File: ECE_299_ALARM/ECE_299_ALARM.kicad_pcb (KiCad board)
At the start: 2 copper layers, 60 x 50 mm, 16 parts, among them SW1 SW_Push_Dual, SW2 SW_Push_Dual, SW3 SW_Push_Dual, SW4 SW_Push_Dual, U1 RDA5807M_Module, U2 RPi_Pico_TH, U3 LM386

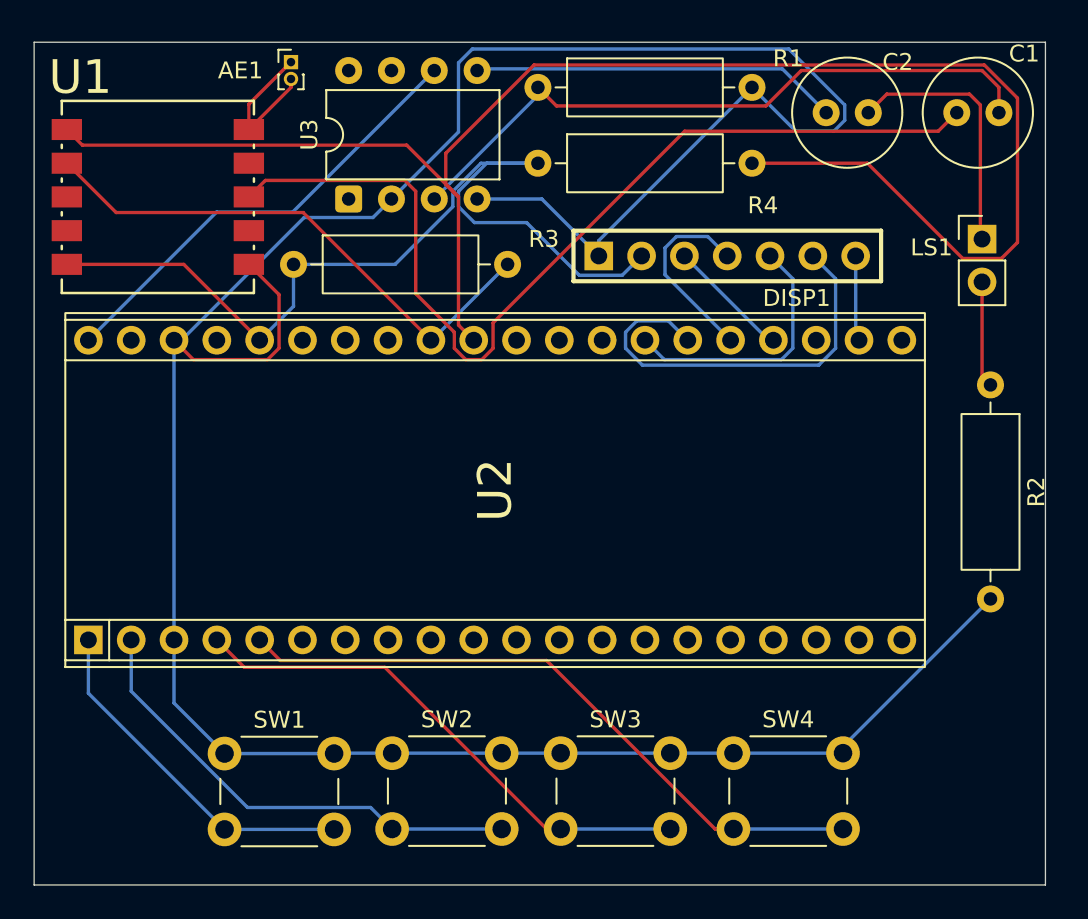
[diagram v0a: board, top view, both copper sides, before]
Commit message: added pcb files
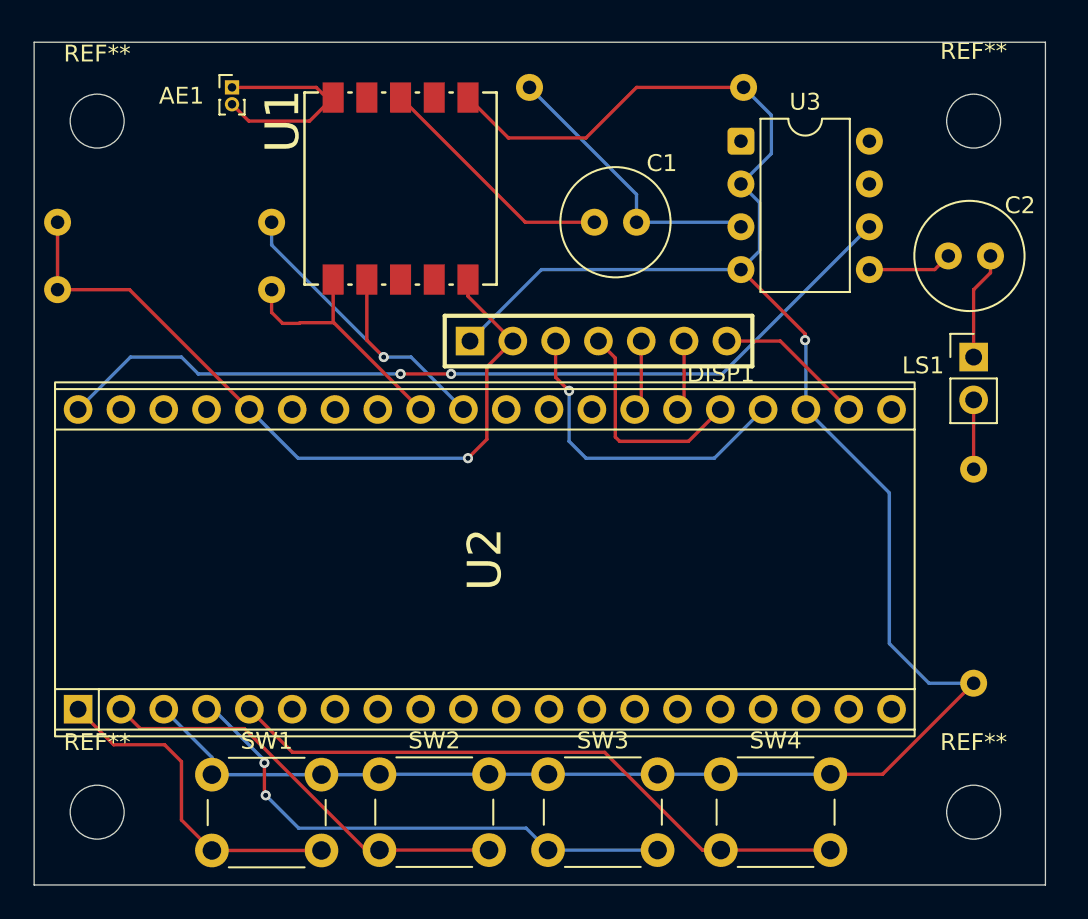
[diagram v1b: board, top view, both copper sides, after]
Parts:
- added REF**: MountingHole_3.2mm_M3, MountingHole:MountingHole_3.2mm_M3, F.Cu at (90.0, 115.0)
- added REF**: MountingHole_3.2mm_M3, MountingHole:MountingHole_3.2mm_M3, F.Cu at (142.0, 115.0)
- added REF**: MountingHole_3.2mm_M3, MountingHole:MountingHole_3.2mm_M3, F.Cu at (142.0, 74.0)
- added REF**: MountingHole_3.2mm_M3, MountingHole:MountingHole_3.2mm_M3, F.Cu at (90.0, 74.0)
- R1, R2, R3, R4: moved to B.Cu
- moved R4 28.7 mm to (87.7, 80.0)
- moved U3 23.5 mm to (128.2, 75.2), turned to 0 degrees
- moved C1 22.5 mm to (119.5, 80.0)
- moved U1 14.4 mm to (108.0, 78.0), turned to 90 degrees
- moved R3 14.1 mm to (87.7, 84.0)
- moved C2 11.2 mm to (140.5, 82.0)
- moved DISP1 9.16 mm to (102.0, 119.0)
- moved LS1 7.02 mm to (142.0, 88.0)
- moved R2 5.10 mm to (142.0, 94.7)
- moved U2 4.16 mm to (113.0, 100.0)
- moved AE1 3.81 mm to (98.0, 72.0)
- moved SW1 1.46 mm to (96.8, 112.8)
- moved SW2 1.46 mm to (106.8, 112.8)
- moved SW3 1.46 mm to (116.8, 112.8)
- moved SW4 1.46 mm to (127.0, 112.8)
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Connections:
- R3 pad 2: Net-(U1-SCLK) -> Net-(U1-SDIO)
- R4 pad 2: Net-(U1-SDIO) -> Net-(U1-SCLK)
- U2 pad 23: unconnected-(U2-GND-Pad23) -> GND
- U2 pad 31: Net-(U1-SDIO) -> Net-(U1-SCLK)
- U2 pad 32: Net-(U1-SCLK) -> Net-(U1-SDIO)
- U2 pad 38: GND -> unconnected-(U2-GND-Pad38)
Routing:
- net Net-(U1-SDIO): track 100.6 -> 15.2 mm
- net Net-(U1-LOUT): track 57.9 -> 14.6 mm
- net GND: track 168.8 -> 133.9 mm, vias 0 -> 1
- net +5V: track 27.1 -> 52.3 mm, vias 0 -> 2
- net Net-(U3-+): track 40.8 -> 16.9 mm
- net Net-(DISP1-DC): track 24.7 -> 4.22 mm
- net Net-(C2-Pad1): track 21.8 -> 5.02 mm
- net Net-(DISP1-SCLK): track 7.35 -> 19.4 mm, vias 0 -> 1
- net Net-(DISP1-RES): track 15.6 -> 4.22 mm
- net Net-(U1-SCLK): track 32.4 -> 21.8 mm, vias 0 -> 1
- net +3.3V: track 55.5 -> 45.3 mm, vias 0 -> 1
- net Net-(C2-Pad2): track 15.4 -> 6.41 mm
- net Net-(U1-FMIN): track 9.07 -> 13.2 mm
- net Net-(DISP1-CS): track 5.08 -> 8.91 mm
- net SW2: track 28.4 -> 25.3 mm
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
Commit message: Revert "Web app"
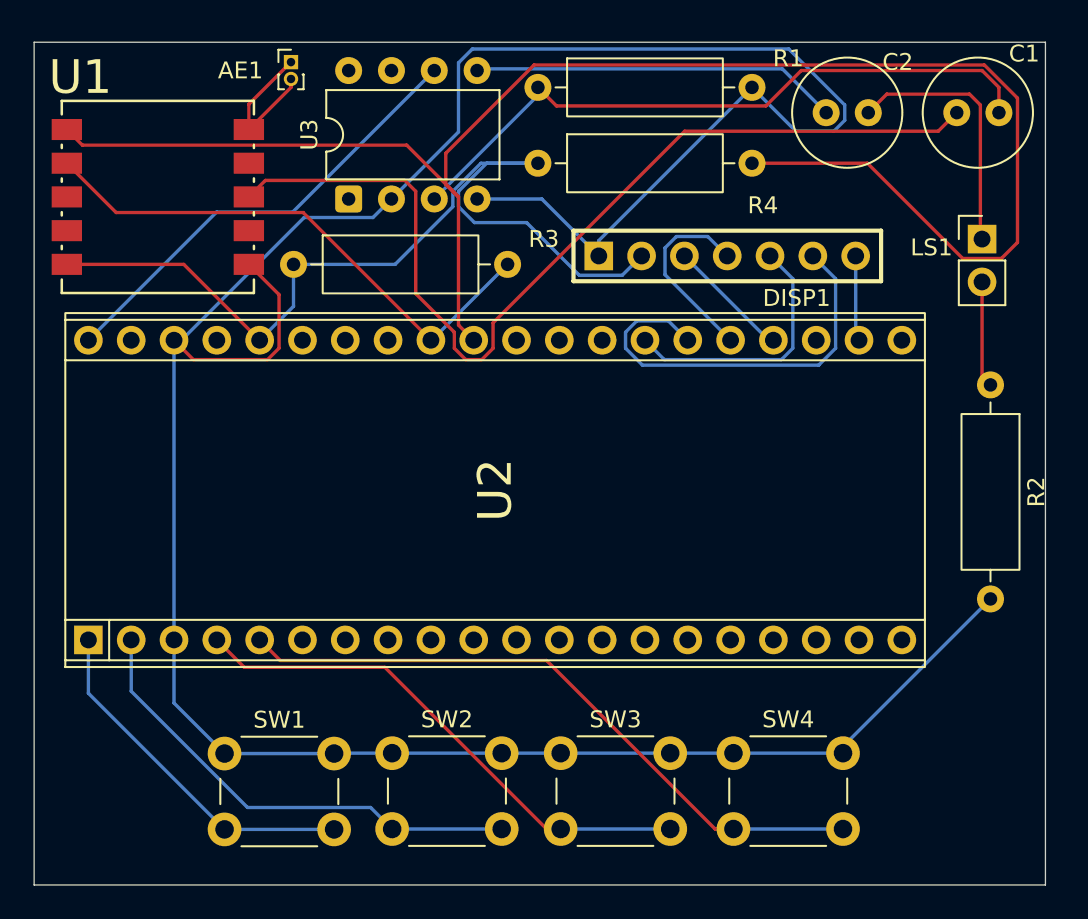
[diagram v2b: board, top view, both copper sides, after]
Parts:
- removed REF** (x4): MountingHole_3.2mm_M3, MountingHole:MountingHole_3.2mm_M3
- R1, R2, R3, R4: moved to F.Cu
- moved R4 28.7 mm to (116.2, 76.5)
- moved U3 23.5 mm to (104.9, 78.6), turned to 90 degrees
- moved C1 22.5 mm to (141.0, 73.5)
- moved U1 14.4 mm to (93.6, 78.5), turned to 0 degrees
- moved R3 14.1 mm to (101.7, 82.5)
- moved C2 11.2 mm to (133.2, 73.5)
- moved DISP1 9.16 mm to (109.6, 114.0)
- moved LS1 7.02 mm to (142.5, 81.0)
- moved R2 5.10 mm to (143.0, 89.7)
- moved U2 4.16 mm to (113.6, 95.9)
- moved AE1 3.81 mm to (101.5, 70.5)
- moved SW1 1.46 mm to (97.6, 111.5)
- moved SW2 1.46 mm to (107.5, 111.5)
- moved SW3 1.46 mm to (117.5, 111.5)
- moved SW4 1.46 mm to (127.8, 111.5)
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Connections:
- R3 pad 2: Net-(U1-SDIO) -> Net-(U1-SCLK)
- R4 pad 2: Net-(U1-SCLK) -> Net-(U1-SDIO)
- U2 pad 23: GND -> unconnected-(U2-GND-Pad23)
- U2 pad 31: Net-(U1-SCLK) -> Net-(U1-SDIO)
- U2 pad 32: Net-(U1-SDIO) -> Net-(U1-SCLK)
- U2 pad 38: unconnected-(U2-GND-Pad38) -> GND
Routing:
- net Net-(U1-SDIO): track 15.2 -> 100.6 mm
- net Net-(U1-LOUT): track 14.6 -> 57.9 mm
- net GND: track 133.9 -> 168.8 mm, vias 1 -> 0
- net +5V: track 52.3 -> 27.1 mm, vias 2 -> 0
- net Net-(U3-+): track 16.9 -> 40.8 mm
- net Net-(DISP1-DC): track 4.22 -> 24.7 mm
- net Net-(C2-Pad1): track 5.02 -> 21.8 mm
- net Net-(DISP1-SCLK): track 19.4 -> 7.35 mm, vias 1 -> 0
- net Net-(DISP1-RES): track 4.22 -> 15.6 mm
- net Net-(U1-SCLK): track 21.8 -> 32.4 mm, vias 1 -> 0
- net +3.3V: track 45.3 -> 55.5 mm, vias 1 -> 0
- net Net-(C2-Pad2): track 6.41 -> 15.4 mm
- net Net-(U1-FMIN): track 13.2 -> 9.07 mm
- net Net-(DISP1-CS): track 8.91 -> 5.08 mm
- net SW2: track 25.3 -> 28.4 mm
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
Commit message: Add files via upload
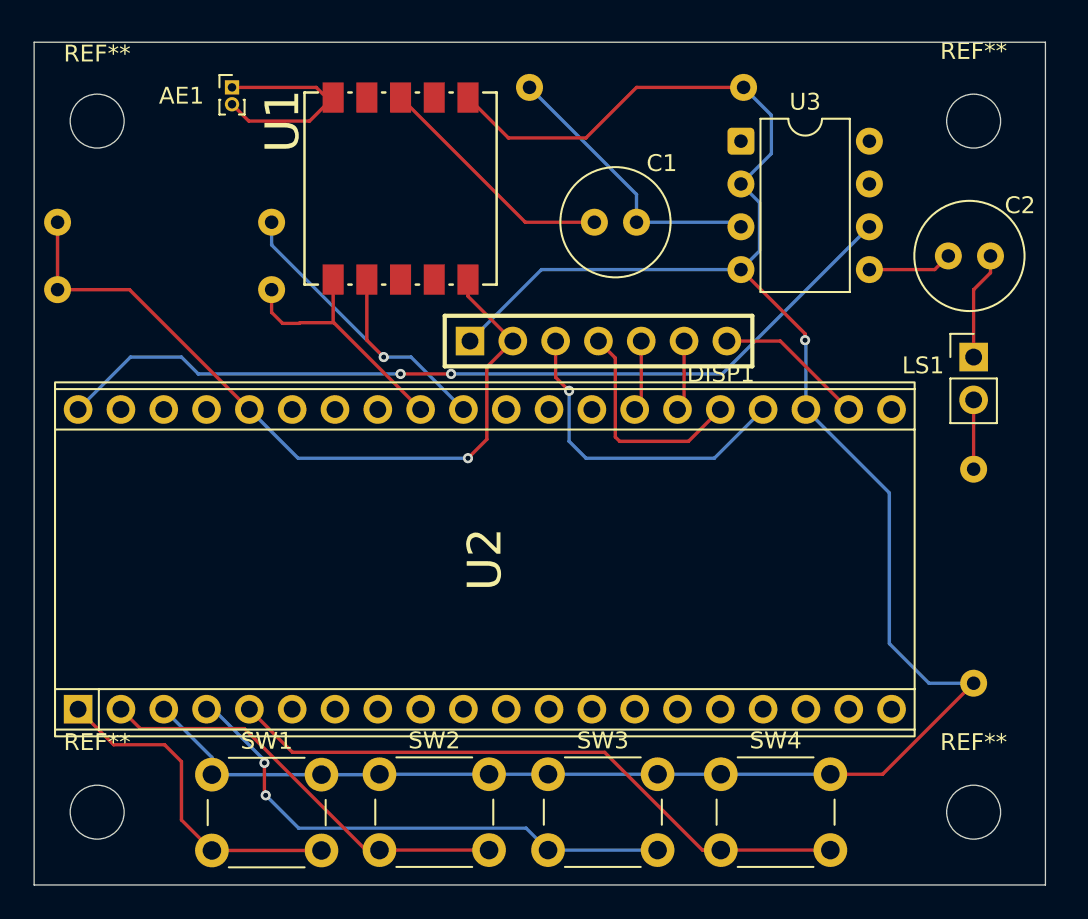
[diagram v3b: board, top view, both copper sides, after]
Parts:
- added REF**: MountingHole_3.2mm_M3, MountingHole:MountingHole_3.2mm_M3, F.Cu at (90.0, 115.0)
- added REF**: MountingHole_3.2mm_M3, MountingHole:MountingHole_3.2mm_M3, F.Cu at (142.0, 115.0)
- added REF**: MountingHole_3.2mm_M3, MountingHole:MountingHole_3.2mm_M3, F.Cu at (142.0, 74.0)
- added REF**: MountingHole_3.2mm_M3, MountingHole:MountingHole_3.2mm_M3, F.Cu at (90.0, 74.0)
- R1, R2, R3, R4: moved to B.Cu
- moved R4 28.7 mm to (87.7, 80.0)
- moved U3 23.5 mm to (128.2, 75.2), turned to 0 degrees
- moved C1 22.5 mm to (119.5, 80.0)
- moved U1 14.4 mm to (108.0, 78.0), turned to 90 degrees
- moved R3 14.1 mm to (87.7, 84.0)
- moved C2 11.2 mm to (140.5, 82.0)
- moved DISP1 9.16 mm to (102.0, 119.0)
- moved LS1 7.02 mm to (142.0, 88.0)
- moved R2 5.10 mm to (142.0, 94.7)
- moved U2 4.16 mm to (113.0, 100.0)
- moved AE1 3.81 mm to (98.0, 72.0)
- moved SW1 1.46 mm to (96.8, 112.8)
- moved SW2 1.46 mm to (106.8, 112.8)
- moved SW3 1.46 mm to (116.8, 112.8)
- moved SW4 1.46 mm to (127.0, 112.8)
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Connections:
- R3 pad 2: Net-(U1-SCLK) -> Net-(U1-SDIO)
- R4 pad 2: Net-(U1-SDIO) -> Net-(U1-SCLK)
- U2 pad 23: unconnected-(U2-GND-Pad23) -> GND
- U2 pad 31: Net-(U1-SDIO) -> Net-(U1-SCLK)
- U2 pad 32: Net-(U1-SCLK) -> Net-(U1-SDIO)
- U2 pad 38: GND -> unconnected-(U2-GND-Pad38)
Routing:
- net Net-(U1-SDIO): track 100.6 -> 15.2 mm
- net Net-(U1-LOUT): track 57.9 -> 14.6 mm
- net GND: track 168.8 -> 133.9 mm, vias 0 -> 1
- net +5V: track 27.1 -> 52.3 mm, vias 0 -> 2
- net Net-(U3-+): track 40.8 -> 16.9 mm
- net Net-(DISP1-DC): track 24.7 -> 4.22 mm
- net Net-(C2-Pad1): track 21.8 -> 5.02 mm
- net Net-(DISP1-SCLK): track 7.35 -> 19.4 mm, vias 0 -> 1
- net Net-(DISP1-RES): track 15.6 -> 4.22 mm
- net Net-(U1-SCLK): track 32.4 -> 21.8 mm, vias 0 -> 1
- net +3.3V: track 55.5 -> 45.3 mm, vias 0 -> 1
- net Net-(C2-Pad2): track 15.4 -> 6.41 mm
- net Net-(U1-FMIN): track 9.07 -> 13.2 mm
- net Net-(DISP1-CS): track 5.08 -> 8.91 mm
- net SW2: track 28.4 -> 25.3 mm
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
